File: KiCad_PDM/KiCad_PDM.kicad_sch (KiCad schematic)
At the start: 0 parts

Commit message: initial commit
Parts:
- added C1, C2: 1uF, symbol Device:C
- added C3: 2.2nF, symbol Device:C
- added C4: 10nF, symbol Device:C
- added D1, D4: MMSZ47202T1G, Diode_SMD:D_SOD-123, symbol PDM:onsemi MMSZ4702T1G
- added D2, D3: FR107, Diode_SMD:D_SOD-123, symbol PDM:JSMSEMI FR107
- added J1: 6437288-1, 6437288-1, symbol 6437288-1:6437288-1
- added R1: 39K, symbol Device:R
- added R2: 1K, symbol Device:R
- added R3: 5.1K, symbol Device:R
- added R4: 50, symbol Device:R
- added U1: NSG2000, Package_SO:SOP-8_3.76x4.96mm_P1.27mm, symbol PDM:NSG2000
- added U2: 2N7002, Package_TO_SOT_SMD:SOT-23_Handsoldering, symbol PDM:Nexperia 2N7002BK,215
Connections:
- new net: D4.1, R3.2, R4.1
- new net: C4.1, R4.2
- new net: C3.1, R1.2, R2.1, U1.3 (Osc)
- new net: R2.2, U2.3
- new net: C2.1, D1.1, D2.1, U1.8 (BST)
- new net: C2.2, D1.2, D3.2, U1.6 (TS)
- new net: R3.1, U2.1
- new net: D2.2, D3.1
- new net +BATT: C1.1, R1.1, U1.1 (VCC)
- new net Ch1: U1.2 (In)
- new net GND: C1.2, C3.2, D4.2, U1.4 (GND), U2.2

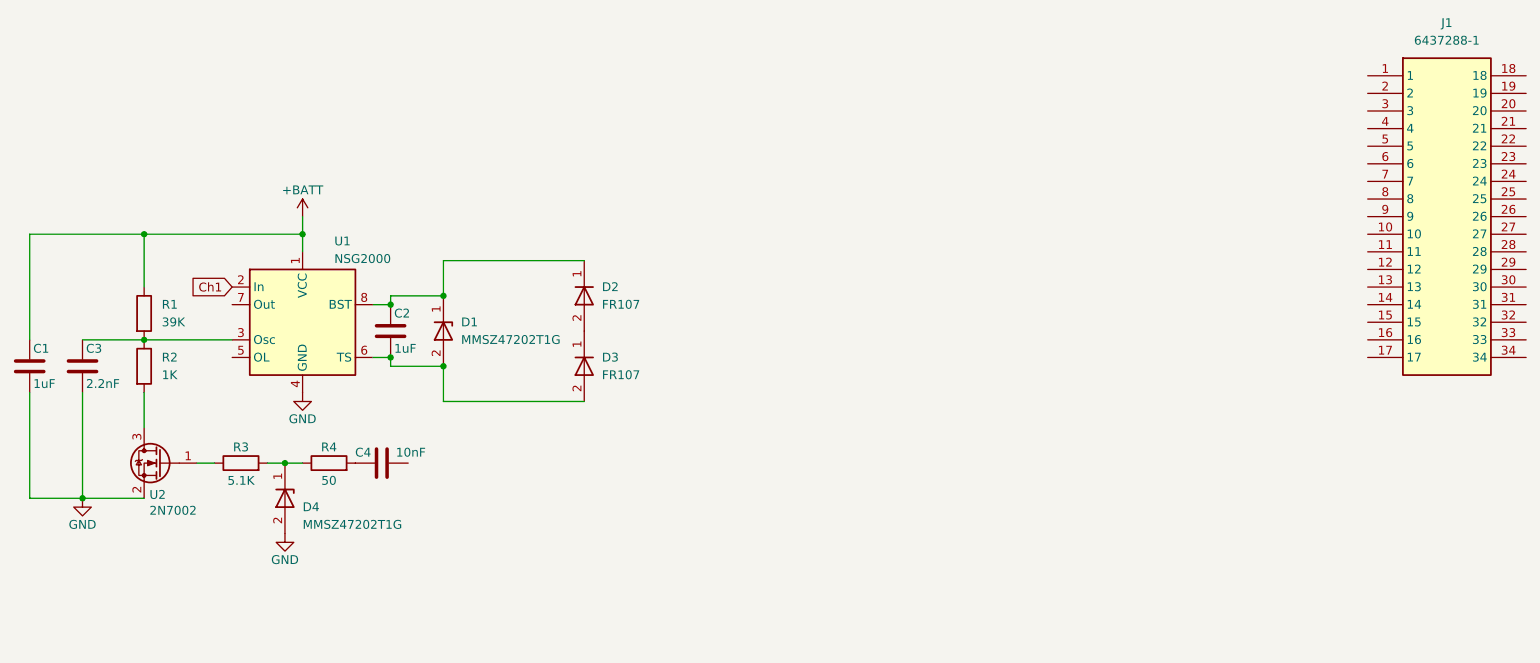
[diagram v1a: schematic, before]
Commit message: initial commit
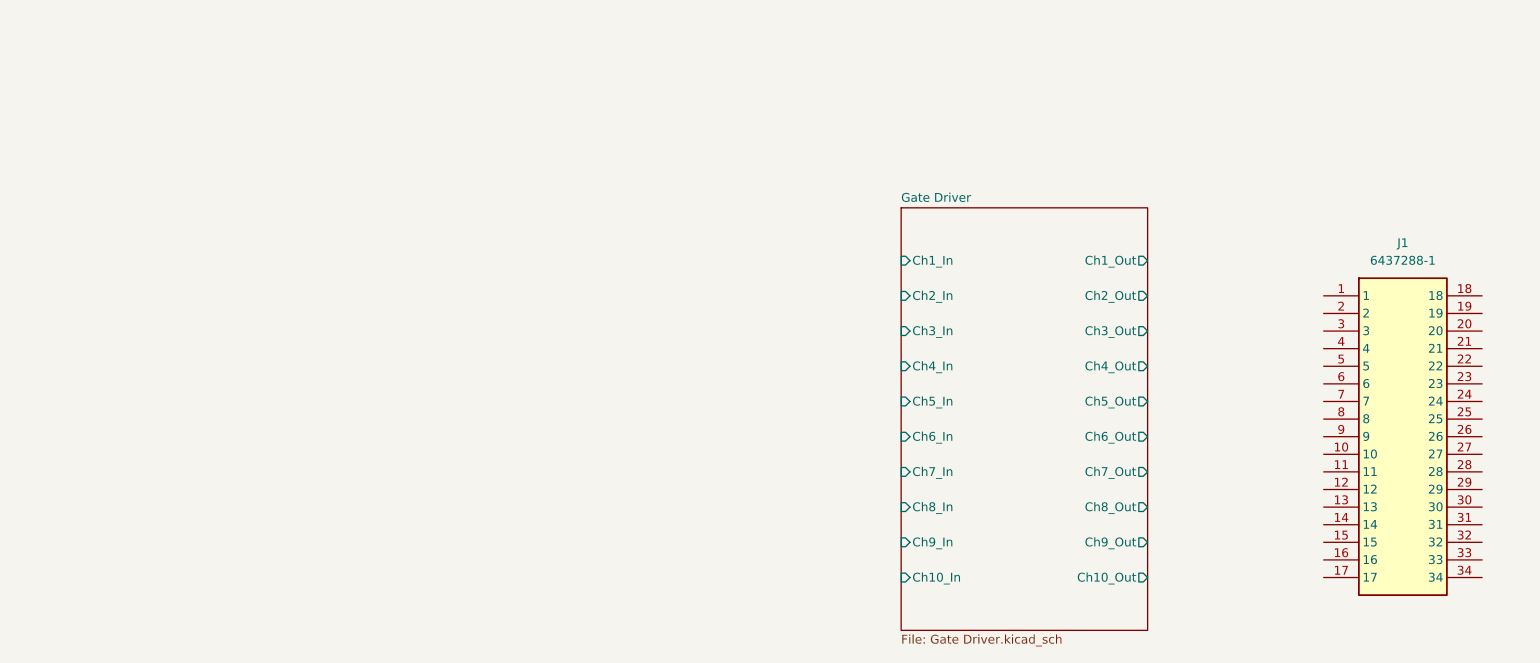
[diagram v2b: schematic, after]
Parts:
- removed C1, C2: 1uF, symbol Device:C
- removed C3: 2.2nF, symbol Device:C
- removed C4: 10nF, symbol Device:C
- removed D1, D4: MMSZ47202T1G, Diode_SMD:D_SOD-123, symbol PDM:onsemi MMSZ4702T1G
- removed D2, D3: FR107, Diode_SMD:D_SOD-123, symbol PDM:JSMSEMI FR107
- removed R1: 39K, symbol Device:R
- removed R2: 1K, symbol Device:R
- removed R3: 5.1K, symbol Device:R
- removed R4: 50, symbol Device:R
- removed U1: NSG2000, Package_SO:SOP-8_3.76x4.96mm_P1.27mm, symbol PDM:NSG2000
- removed U2: 2N7002, Package_TO_SOT_SMD:SOT-23_Handsoldering, symbol PDM:Nexperia 2N7002BK,215
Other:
- added sheet Gate Driver (Gate Driver.kicad_sch)
- moved on the sheet: J1
